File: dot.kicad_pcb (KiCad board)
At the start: 2 copper layers, 93 x 55 mm, 61 parts, among them J1 PWR, J2 GPIO, J3 EX_SERIAL, J4 USB_C_Receptacle_USB2.0, J5 Micro_SD_Card_Det, J6 STRIP0, J7 STRIP1, J8 STRIP2, J9 STRIP3, Q1 SQM40031EL, Q2 MMBT2222, Q3 MMBT2222, SW1 SW_Push, SW2 BLE, SW3 CONFIG_RST, SW4 USER, U1 ESP32-WROOM-32D, U2 ADP2108AUJ-3.3, U3 CP2104, U4 TXB0104D

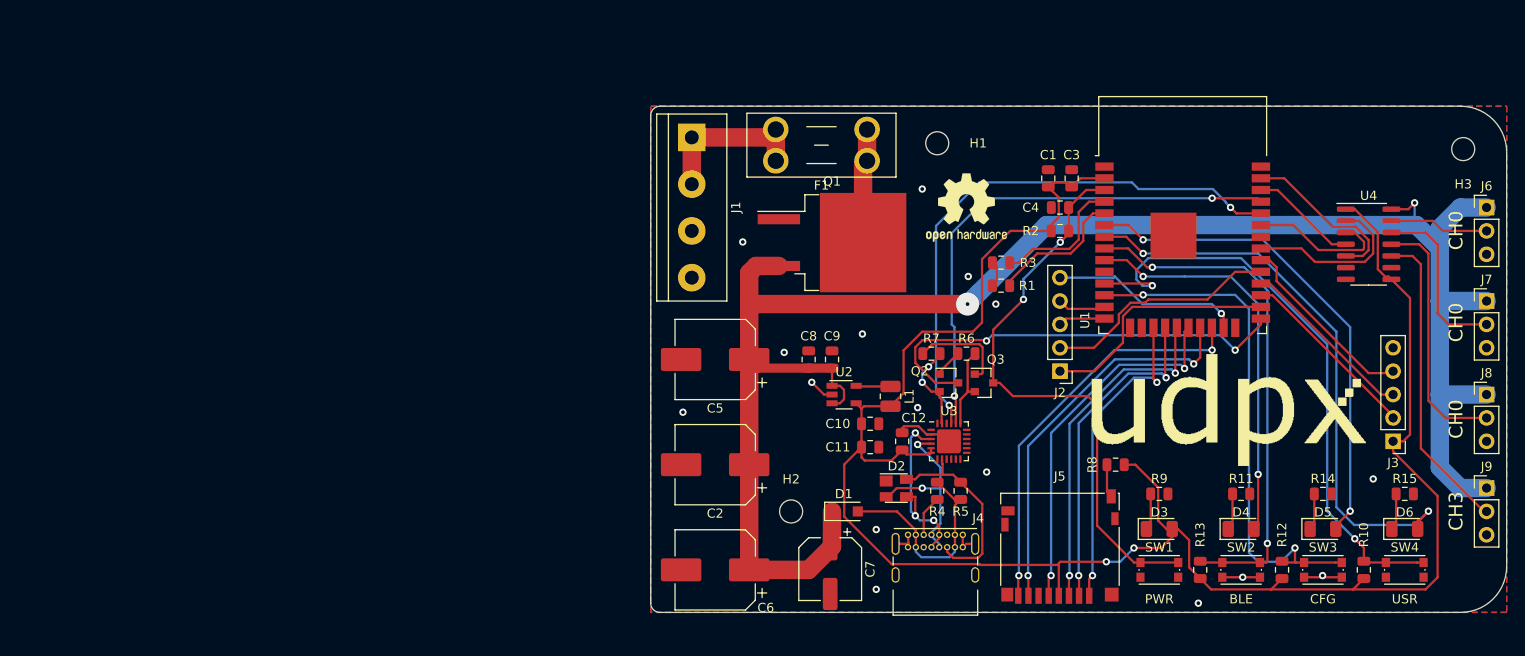
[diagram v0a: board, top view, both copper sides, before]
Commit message: Ordered files
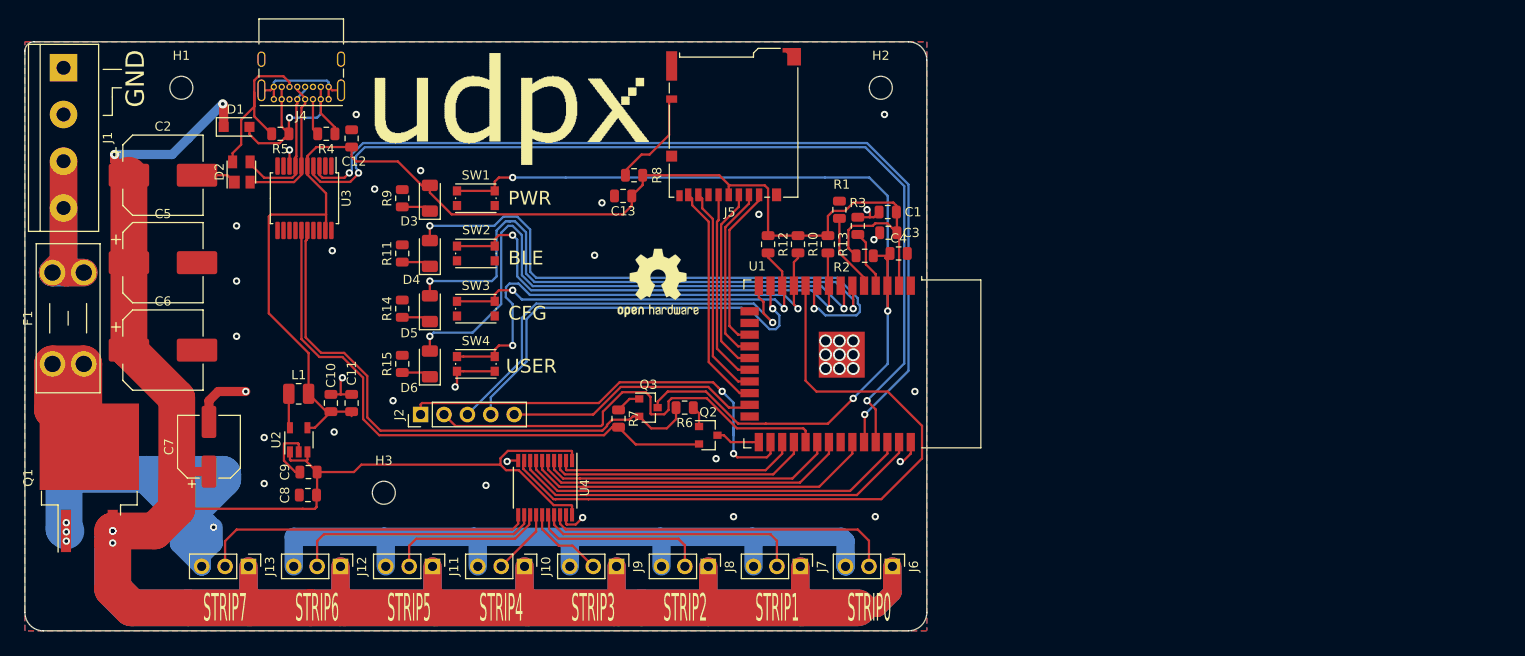
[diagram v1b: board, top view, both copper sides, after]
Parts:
- removed J3: EX_SERIAL, Connector_PinHeader_2.54mm:PinHeader_1x05_P2.54mm_Vertical
- removed the REF** at (203.2, 118.1)
- added C13: 1uF, Capacitor_SMD:C_0805_2012Metric, F.Cu at (117.0, 78.8)
- added J10: STRIP4, Connector_PinHeader_2.54mm:PinHeader_1x03_P2.54mm_Vertical, F.Cu at (106.3, 119.0)
- added J11: STRIP5, Connector_PinHeader_2.54mm:PinHeader_1x03_P2.54mm_Vertical, F.Cu at (96.3, 119.0)
- added J12: STRIP6, Connector_PinHeader_2.54mm:PinHeader_1x03_P2.54mm_Vertical, F.Cu at (86.3, 119.0)
- added J13: STRIP7, Connector_PinHeader_2.54mm:PinHeader_1x03_P2.54mm_Vertical, F.Cu at (76.3, 119.0)
- J5: footprint Connector_Card:microSD_HC_Hirose_DM3D-SF -> Connector_Card:microSD_HC_Hirose_DM3BT-DSF-PEJS
- U3: value CP2104 -> CH340T; footprint Package_DFN_QFN:QFN-24-1EP_4x4mm_P0.5mm_EP2.6x2.6mm -> Package_SO:SSOP-20_5.3x7.2mm_P0.65mm
- U4: value TXB0104D -> 74HCT245; footprint Package_SO:SOIC-14_3.9x8.7mm_P1.27mm -> Package_SO:TSSOP-20_4.4x6.5mm_P0.65mm
- moved H3 123.1 mm to (91.0, 111.0), turned to 0 degrees
- moved R15 109.8 mm to (93.0, 97.0), turned to 90 degrees
- moved D6 107.4 mm to (96.0, 97.0), turned to 90 degrees
- moved SW4 103.4 mm to (101.0, 97.0)
- moved R14 102.0 mm to (93.0, 91.0), turned to 90 degrees
- moved D5 99.9 mm to (96.0, 91.0), turned to 90 degrees
- moved SW3 96.3 mm to (101.0, 91.0)
- moved J9 94.9 mm to (116.3, 119.0), turned to 270 degrees
- moved R11 94.8 mm to (93.0, 85.0), turned to 90 degrees
- moved U4 93.3 mm to (108.5, 110.5), turned to 270 degrees
- moved D4 93.1 mm to (96.0, 85.0), turned to 90 degrees
- moved F1 91.2 mm to (55.0, 97.0), turned to 90 degrees
- moved SW2 90.0 mm to (101.0, 85.0)
- moved R9 88.3 mm to (93.0, 79.0), turned to 90 degrees
- moved D3 87.0 mm to (96.0, 79.0), turned to 90 degrees
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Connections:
- J1 pad 1: Net-(F1-Pad2) -> GND
- J1 pad 2: Net-(F1-Pad2) -> GND
- J1 pad 3: GND -> Net-(F1-Pad2)
- J1 pad 4: GND -> Net-(F1-Pad2)
- J4 pad A8: Net-(J4-PadA8) -> (no net)
- J4 pad B8: Net-(J4-PadB8) -> (no net)
- U1 pad 10: Net-(U1-Pad10) -> /STRIP0
- U1 pad 16: Net-(U1-Pad16) -> (no net)
- U1 pad 24: Net-(U1-Pad24) -> (no net)
- U1 pad 27: /EX_RX -> /STRIP7
- U1 pad 28: /EX_TX -> /STRIP6
- U1 pad 30: /EX_IRQ -> /STRIP5
- U1 pad 31: /STRIP0 -> /STRIP4
- U1 pad 32: Net-(U1-Pad32) -> (no net)
- U1 pad 33: /STRIP1 -> /STRIP3
- U1 pad 37: /STRIP3 -> /STRIP1
- U3 pad 1: Net-(U3-Pad1) -> (no net)
- U3 pad 10: Net-(U3-Pad10) -> (no net)
- U3 pad 11: Net-(U3-Pad11) -> (no net)
- U3 pad 12: Net-(U3-Pad12) -> (no net)
- U3 pad 13: Net-(U3-Pad13) -> (no net)
- U3 pad 14: Net-(U3-Pad14) -> (no net)
- U3 pad 15: Net-(U3-Pad15) -> /DTR
- U3 pad 16: Net-(U3-Pad16) -> /RTS
- U3 pad 17: Net-(U3-Pad17) -> (no net)
- U3 pad 18: Net-(U3-Pad18) -> (no net)
- U3 pad 19: /RTS -> +3V3
- U3 pad 2: GND -> (no net)
- U3 pad 20: /TX -> (no net)
- U3 pad 3: Net-(D2-Pad3) -> /RX
- U3 pad 4: Net-(D2-Pad2) -> /TX
- U3 pad 6: +3V3 -> Net-(D2-Pad2)
- U3 pad 7: Net-(U3-Pad7) -> Net-(D2-Pad3)
- U3 pad 8: Net-(D2-Pad4) -> GND
- U3 pad 9: Net-(U3-Pad9) -> (no net)
- U4 pad 1: +3V3 -> +5V
- U4 pad 10: Net-(J9-Pad2) -> GND
- U4 pad 11: Net-(J8-Pad2) -> Net-(J13-Pad2)
- U4 pad 12: Net-(J7-Pad2) -> Net-(J12-Pad2)
- U4 pad 13: Net-(J6-Pad2) -> Net-(J11-Pad2)
- U4 pad 14: +5V -> Net-(J10-Pad2)
- U4 pad 2: /STRIP0 -> /STRIP7
- U4 pad 3: /STRIP1 -> /STRIP6
- U4 pad 4: /STRIP2 -> /STRIP5
- U4 pad 5: /STRIP3 -> /STRIP4
- U4 pad 6: Net-(U4-Pad6) -> /STRIP3
- U4 pad 7: GND -> /STRIP2
- U4 pad 8: +3V3 -> /STRIP1
- U4 pad 9: Net-(U4-Pad9) -> /STRIP0
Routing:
- net +5V: track 198.2 -> 393.3 mm, vias 2 -> 6
- net GND: track 25.8 -> 191.4 mm, vias 16 -> 42
- net +3V3: track 209.1 -> 144.7 mm, vias 2 -> 0
- net /STRIP0: track 18.8 -> 76.0 mm
- net /DTR: track 9.80 -> 63.1 mm, vias 2 -> 0
- net /RTS: track 9.01 -> 61.7 mm
- net /TX: track 56.2 -> 100.2 mm
- net /GPIO0: track 47.9 -> 4.81 mm, vias 2 -> 0
- net /RESET: track 63.0 -> 105.8 mm, vias 2 -> 3
- net Net-(J2-Pad3): track 5.10 -> 46.3 mm, vias 0 -> 1
- net Net-(J2-Pad4): track 5.28 -> 45.8 mm, vias 0 -> 1
- net /RX: track 60.9 -> 99.5 mm
- net Net-(J13-Pad2): track 0.00 -> 36.4 mm
- net /STRIP4: track 0.00 -> 34.6 mm
- net /STRIP5: track 0.00 -> 32.3 mm
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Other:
- board size 93 x 55 mm -> 98 x 64 mm
- net class Default: clearance 0.2 -> 0.15
- rule trace_clearance: 0.2 -> 0.15
- board text added: "@MartinFasani @IoTPanic @Hputzek"
- board text added: "GND"
- board text added: "Rev 1A"
- board text added: "STRIP0"
- board text added: "STRIP1"
- board text added: "STRIP2"
- board text added: "STRIP3"
- board text added: "STRIP4"
- board text added: "STRIP5"
- board text added: "STRIP6"
- board text added: "STRIP7"
- board text added: "USER"
- board text added: "github.com/IoTPanic/udpx-dot"
- board text removed: "CH0"
- board text removed: "CH3"
- board text removed: "USR"
